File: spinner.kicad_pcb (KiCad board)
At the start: 2 copper layers, 113 parts, among them SW1 SW_SPDT, U1 SFH617A-3X006, U2 SFH617A-3X006, U3 SFH617A-3X006, U4 RS0102, U5 AP63205WU

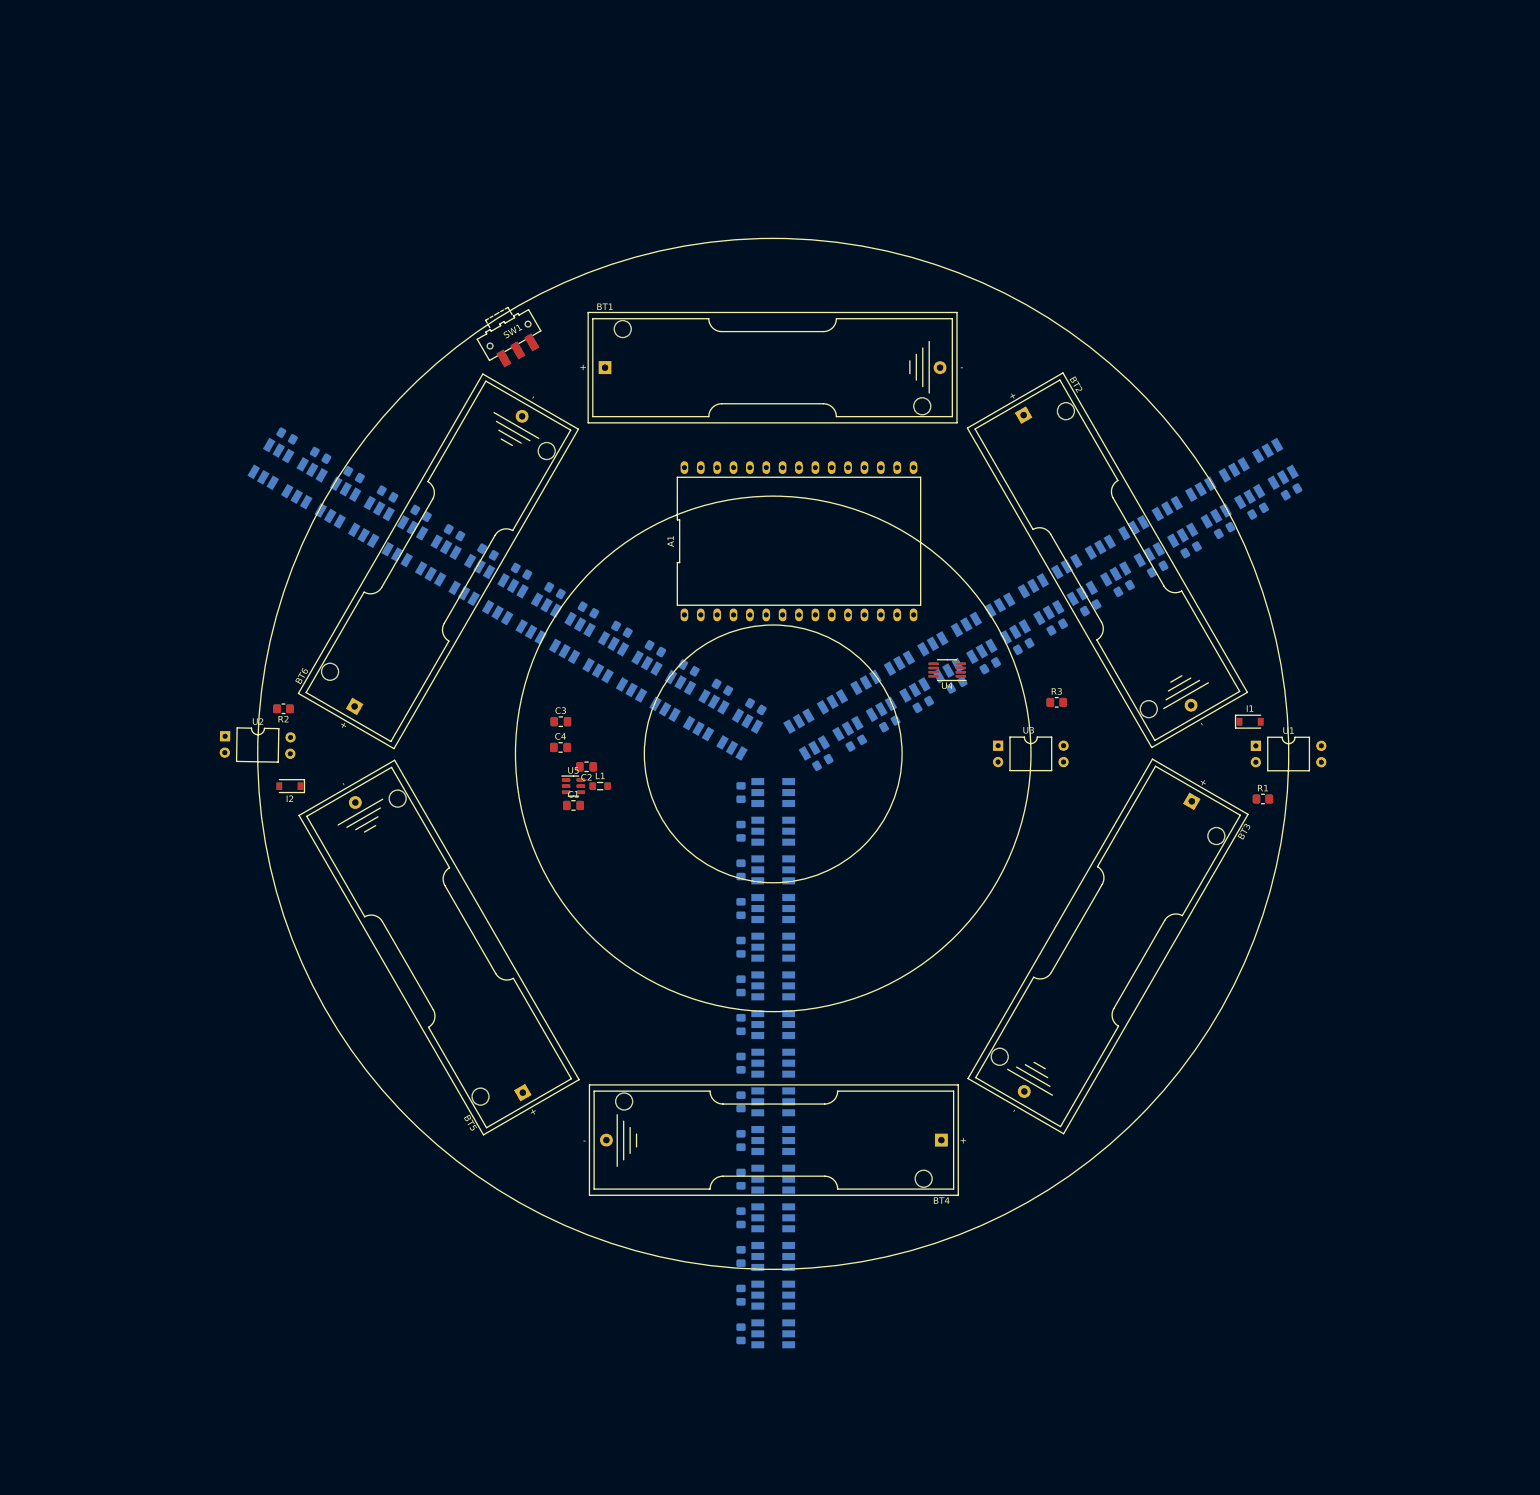
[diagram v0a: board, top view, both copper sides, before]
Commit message: Update things.  Next checkin.
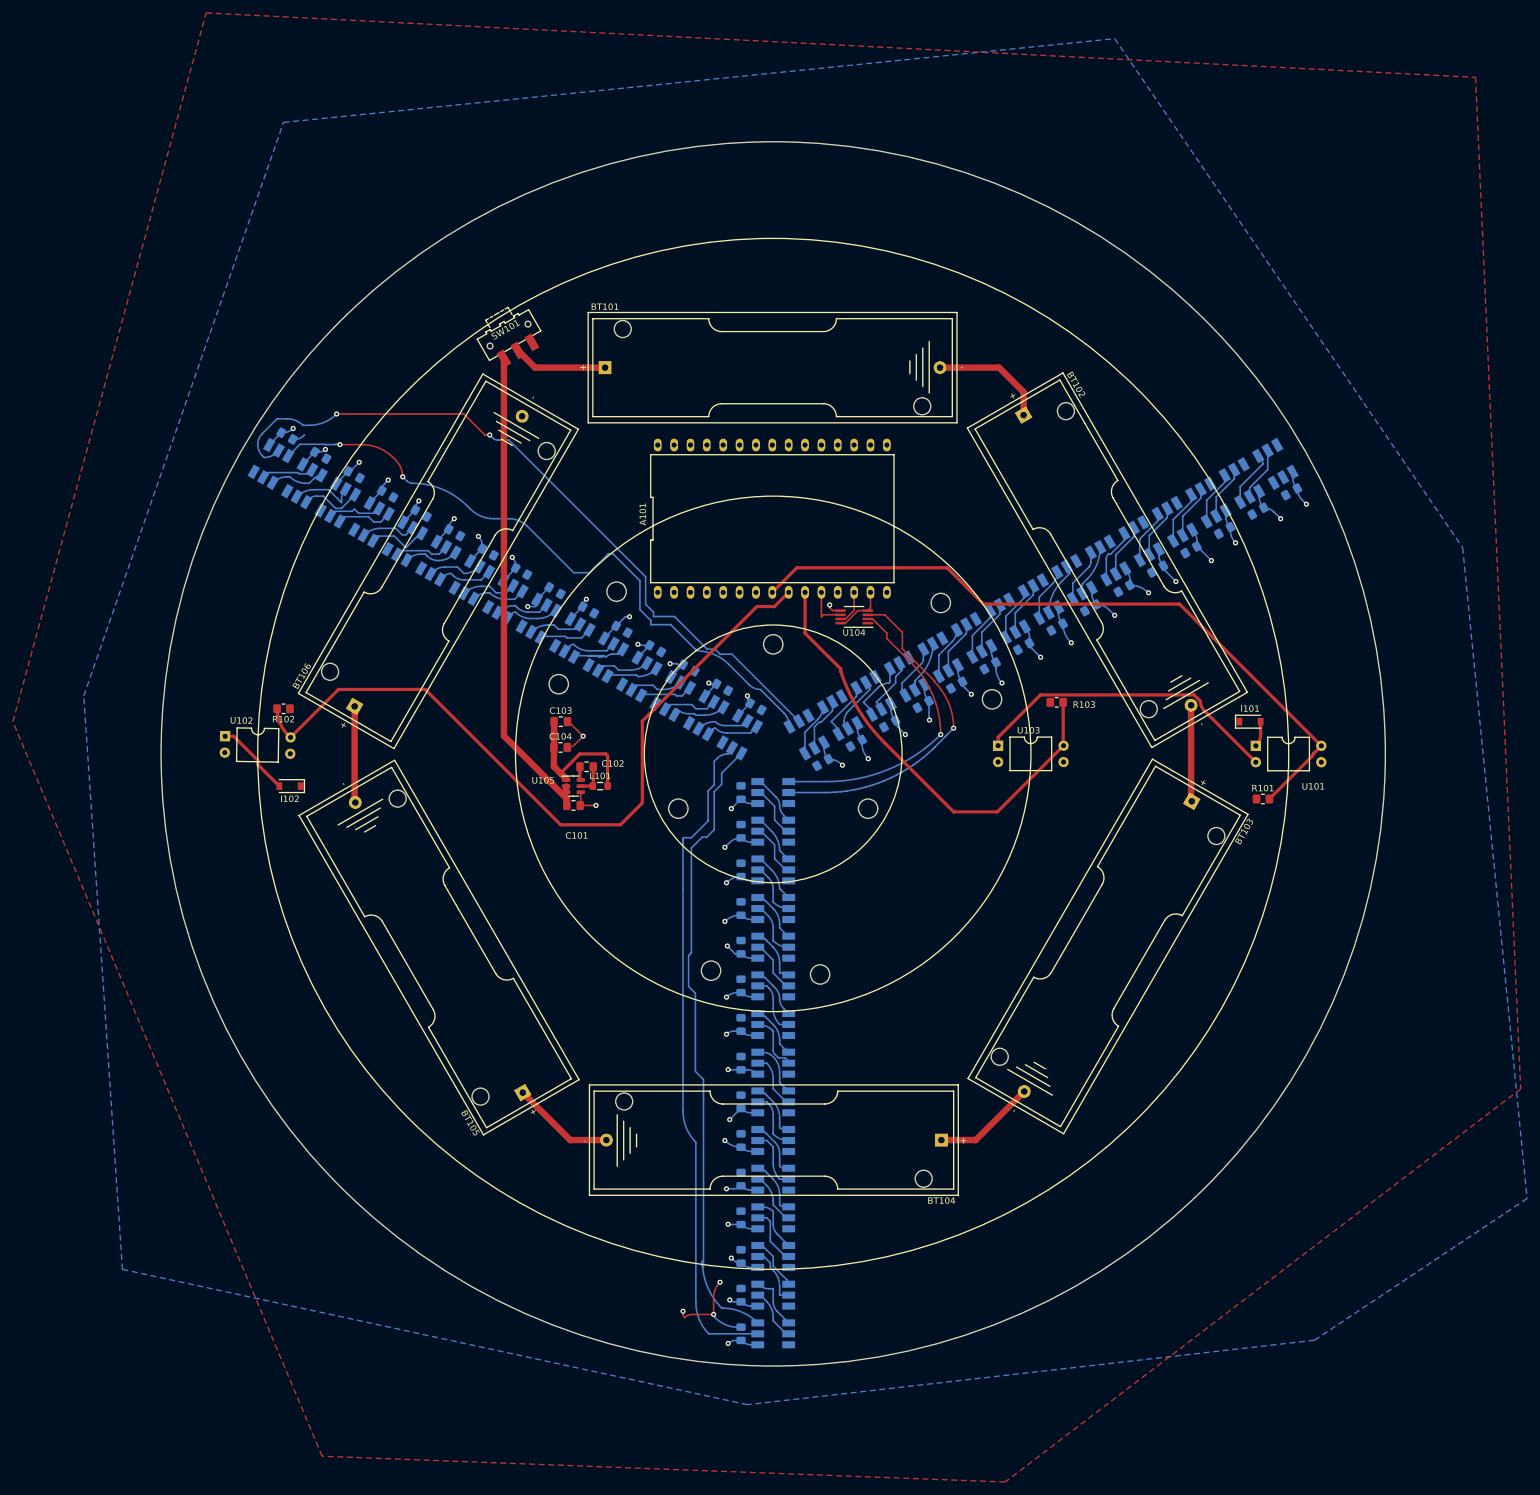
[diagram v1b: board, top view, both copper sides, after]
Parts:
- added H101: MountingHole, MountingHole:MountingHole_3mm, F.Cu at (116.7, 89.2)
- added H102: MountingHole, MountingHole:MountingHole_3mm, F.Cu at (157.3, 134.2)
- added H103: MountingHole, MountingHole:MountingHole_3mm, F.Cu at (135.3, 108.5)
- added H104: MountingHole, MountingHole:MountingHole_3mm, F.Cu at (184.0, 91.5)
- added H105: MountingHole, MountingHole:MountingHole_3mm, F.Cu at (140.4, 133.6)
- added H106: MountingHole, MountingHole:MountingHole_3mm, F.Cu at (176.0, 76.6)
- added H107: MountingHole, MountingHole:MountingHole_3mm, F.Cu at (164.7, 108.5)
- added H108: MountingHole, MountingHole:MountingHole_3mm, F.Cu at (125.7, 74.8)
- added H109: MountingHole, MountingHole:MountingHole_3mm, F.Cu at (150.0, 83.0)
- moved U104 16.6 mm to (162.6, 78.7)
- moved A101 5.42 mm to (149.9, 63.5)
- renumbered A1 to A101, BT1 to BT101, BT2 to BT102, BT3 to BT103, BT4 to BT104, BT5 to BT105, BT6 to BT106, C1 to C101, C2 to C102, C3 to C103, C4 to C104, C301 to C105, C101 to C106, C201 to C107, C302 to C108, C102 to C109, C202 to C110, C303 to C111, C103 to C112, C203 to C113, C304 to C114, C104 to C115, C204 to C116, C305 to C117, C105 to C118, C205 to C119, C306 to C120, C106 to C121, C206 to C122, C307 to C123, C107 to C124, C207 to C125, C308 to C126, C108 to C127, C208 to C128, C309 to C129, C109 to C130, C209 to C131, C310 to C132, C110 to C133, C210 to C134, C311 to C135, C111 to C136, C211 to C137, C312 to C138, C112 to C139, C212 to C140, C313 to C141, C113 to C142, C213 to C143, C314 to C144, C114 to C145, C214 to C146, C315 to C147, C115 to C148, C215 to C149, D301 to D101, D101 to D102, D201 to D103, D302 to D104, D102 to D105, D202 to D106, D303 to D107, D103 to D108, D203 to D109, D304 to D110, D104 to D111, D204 to D112, D305 to D113, D105 to D114, D205 to D115, D306 to D116, D106 to D117, D206 to D118, D307 to D119, D107 to D120, D207 to D121, D308 to D122, D108 to D123, D208 to D124, D309 to D125, D109 to D126, D209 to D127, D310 to D128, D110 to D129, D210 to D130, D311 to D131, D111 to D132, D211 to D133, D312 to D134, D112 to D135, D212 to D136, D313 to D137, D113 to D138, D213 to D139, D314 to D140, D114 to D141, D214 to D142, D315 to D143, D115 to D144, D215 to D145, I1 to I101, I2 to I102, L1 to L101, R1 to R101, R2 to R102, R3 to R103, SW1 to SW101, U1 to U101, U2 to U102, U3 to U103, U4 to U104, U5 to U105
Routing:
- net VCC: track 0.00 -> 254.6 mm, vias 0 -> 45
- net /OPTO_in_1: track 0.00 -> 116.5 mm
- net /CO_3: track 0.00 -> 114.3 mm, vias 0 -> 2
- net /OPTO_in_0: track 0.00 -> 109.8 mm
- net /CO_1: track 0.00 -> 104.7 mm
- net /DO_3: track 0.00 -> 101.9 mm, vias 0 -> 2
- net /DO_1: track 0.00 -> 99.6 mm
- net Net-(C101-Pad1): track 0.00 -> 74.3 mm
- net /OPTO_in_2: track 0.00 -> 70.9 mm
- net /CI: track 0.00 -> 52.9 mm, vias 0 -> 1
- net Net-(U101-Pad2): track 0.00 -> 48.7 mm
- net /DI: track 0.00 -> 47.7 mm, vias 0 -> 1
- net GND: track 0.00 -> 31.2 mm, vias 0 -> 6
- net Net-(BT101-Pad2): track 0.00 -> 18.1 mm
- net Net-(BT104-Pad2): track 0.00 -> 16.0 mm
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- added copper zone on B.Cu, net GND
- added copper zone on F.Cu, net VCC
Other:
- board outline added: 190 x 190 mm

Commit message: Adding all kinds of things.
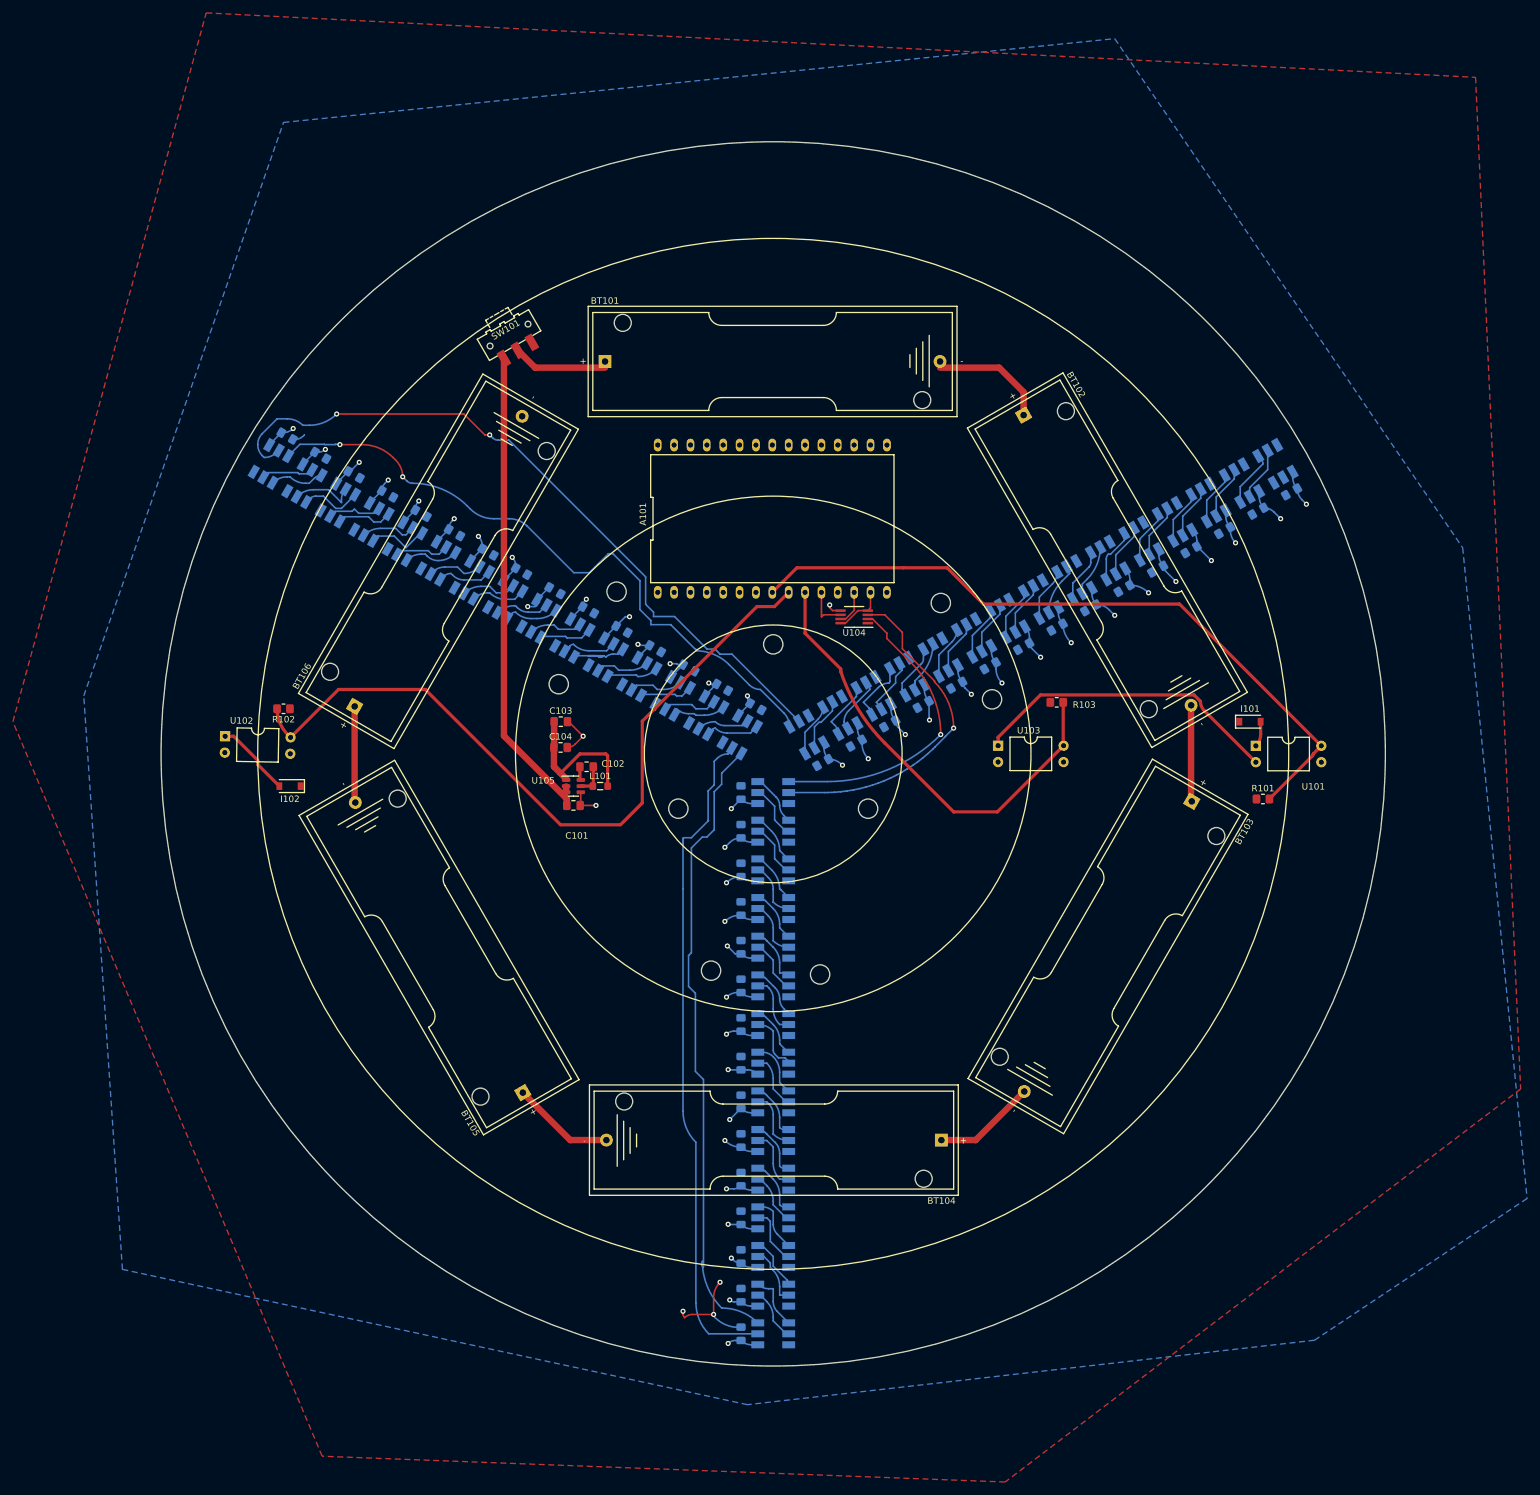
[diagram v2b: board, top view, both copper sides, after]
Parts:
- added G***: LOGO, Library:hakz_04, B.Cu at (152.5, 34.0)
- moved BT101 0.96 mm to (150.0, 39.0)
